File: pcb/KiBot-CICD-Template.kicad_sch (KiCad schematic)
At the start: 1 part

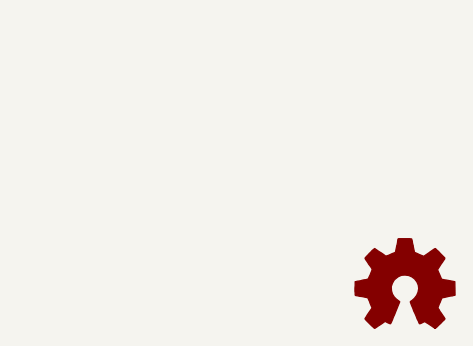
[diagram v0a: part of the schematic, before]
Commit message: update template
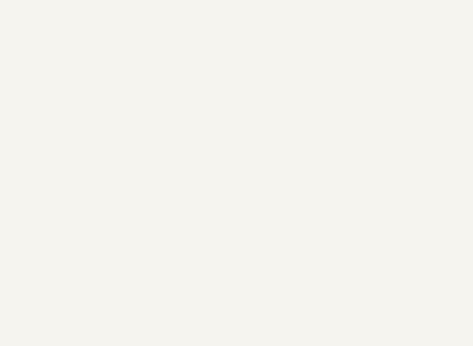
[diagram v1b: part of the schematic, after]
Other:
- company: nerdyscout -> @stop_pattern
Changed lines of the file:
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@@
   (title_block
     (title "KiBot-CICD-Template")
-    (date "${date}")
-    (rev "${version}")
-    (company "nerdyscout")
-    (comment 4 "CERN Open Hardware Licence v2.0")
+    (company "@stop_pattern")
   )
   (wire (pts (xy 99.06 97.79) (xy 99.06 119.38))
@@
   (wire (pts (xy 109.22 119.38) (xy 109.22 114.3))
     (stroke (width 0) (type default) (color 0 0 0 0))
-  )
-  (symbol (lib_id "Graphic:Logo_Open_Hardware_Small") (at 274.32 175.26 0) (unit 1)
-    (in_bom yes) (on_board yes)
-    (property "Reference" "#LOGO1" (id 0) (at 274.32 168.275 0)
-      (effects (font (size 1.27 1.27)) hide)
-    )
-    (property "Value" "Logo_Open_Hardware_Small" (id 1) (at 274.32 180.975 0)
-      (effects (font (size 1.27 1.27)) hide)
-    )
-    (property "Footprint" "Symbol:OSHW-Symbol_6.7x6mm_SilkScreen" (id 2) (at 274.32 175.26 0)
-      (effects (font (size 1.27 1.27)) hide)
-    )
-    (property "Datasheet" "" (id 3) (at 274.32 175.26 0)
-      (effects (font (size 1.27 1.27)) hide)
-    )
   )
   (symbol (lib_id "Device:R") (at 109.22 110.49 0) (unit 1)
@@
   )
   (symbol_instances
-    (path "/00000000-0000-0000-0000-00005e25fd05"
-      (reference "#LOGO1") (unit 1) (value "Logo_Open_Hardware_Small") (footprint "Symbol:OSHW-Symbol_6.7x6mm_SilkScreen")
-    )
     (path "/5f38bdb2-3657-474e-8e86-d6bb0b298110"
       (reference "R1") (unit 1) (value "R") (footprint "")
